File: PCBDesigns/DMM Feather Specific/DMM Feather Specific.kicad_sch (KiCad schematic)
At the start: 63 parts, among them J1 POWER2, J10 I_Input, J11 Conn_01x02_Pin, J12 Conn_01x02_Pin, J2 POWER1, J3 DIGITAL2, J4 Out to Screen, J5 ANALOG, J6 DIGITAL1, J7 Barrel_Jack, J8 Conn_01x01_Socket, J9 Barrel_Jack, Q1 MMBT3904, Q2 AO3400A MOSFET, Q3 AO3400A MOSFET, SW1 SW_Push, SW2 SW_Push, SW3 SW_Push, U1 RFM-0505S, U10 LM4040DBZ-2.5, U11 ADS1115IDGS, U2 ADuM1200AR, U3 ADuM1200AR, U4 ISO1540, U5 LM317_TO-220, U6 LM4040DBZ-5, U7 IX4426N, U8 MAX1683, U9 IX4426N

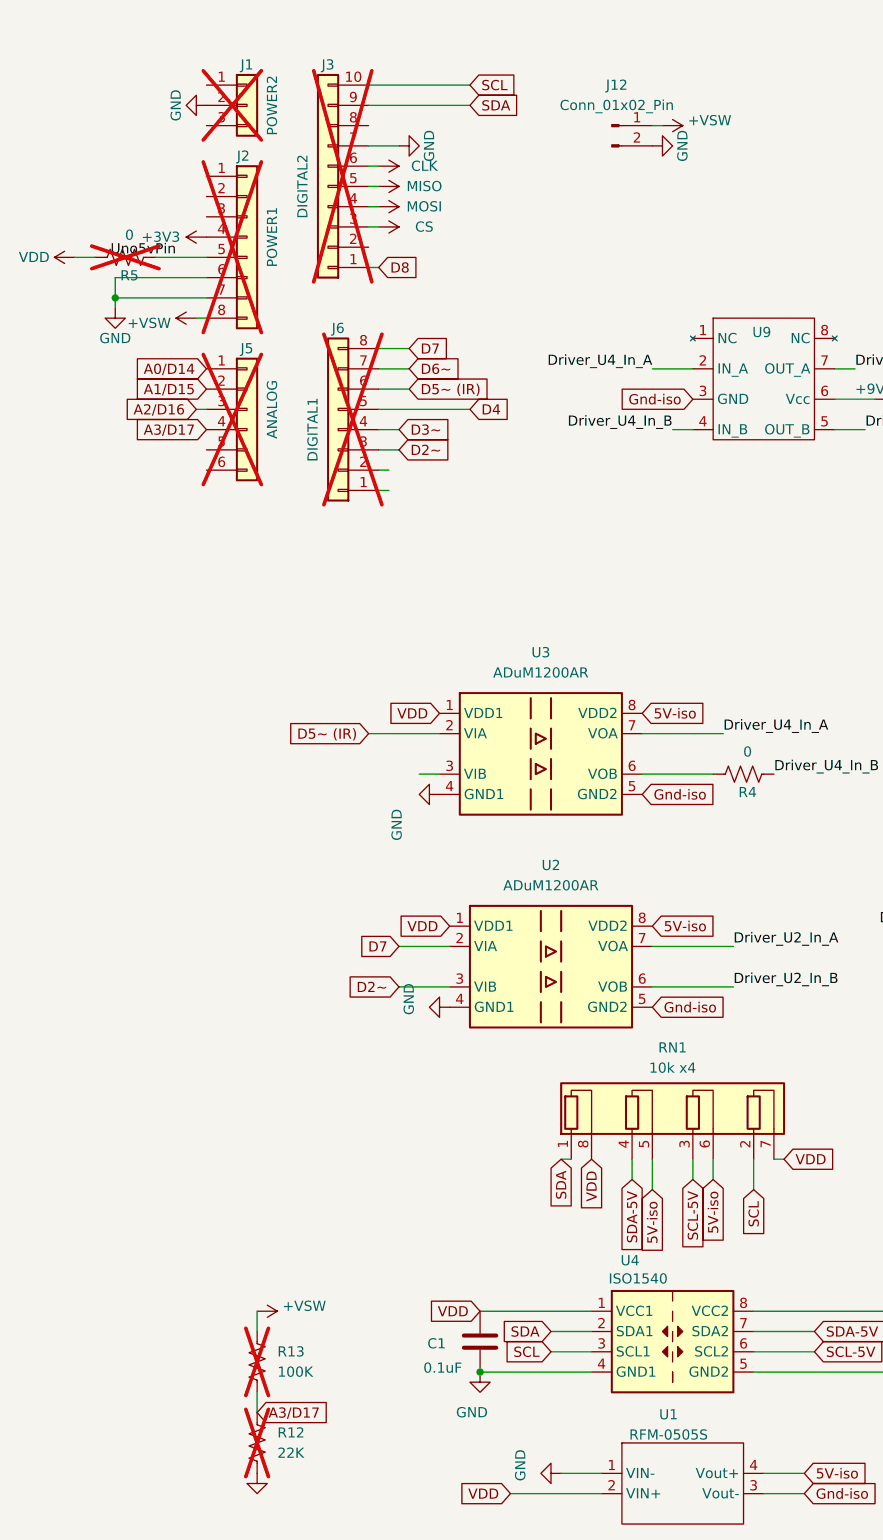
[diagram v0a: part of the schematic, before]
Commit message: Finished(?) an Uno footprint board, started on Feather specific
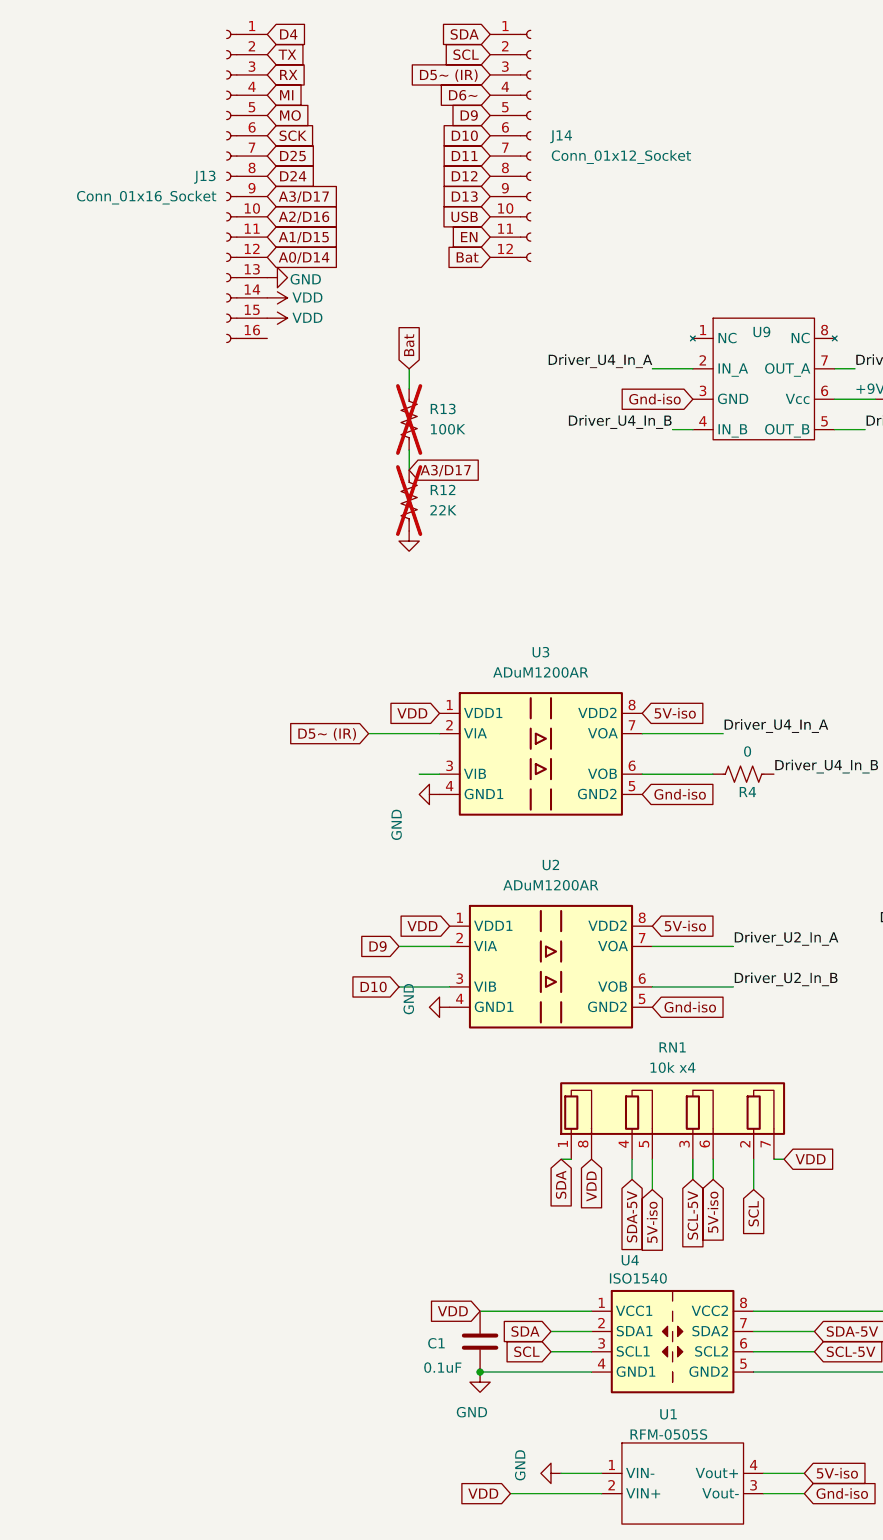
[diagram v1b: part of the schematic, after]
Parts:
- removed J1: POWER2, Library:PinHeader_1x03_P2.54mm_Vertical_NoBox, symbol Connector_Generic:Conn_01x03
- removed J12: Conn_01x02_Pin, Connector_PinSocket_2.54mm:PinSocket_1x02_P2.54mm_Vertical, symbol Connector:Conn_01x02_Pin
- removed J2: POWER1, Connector_PinHeader_2.54mm:PinHeader_1x08_P2.54mm_Vertical, symbol Connector_Generic:Conn_01x08
- removed J3: DIGITAL2, Connector_PinHeader_2.54mm:PinHeader_1x10_P2.54mm_Vertical, symbol Connector_Generic:Conn_01x10
- removed J5: ANALOG, Connector_PinHeader_2.54mm:PinHeader_1x06_P2.54mm_Vertical, symbol Connector_Generic:Conn_01x06
- removed J6: DIGITAL1, Connector_PinHeader_2.54mm:PinHeader_1x08_P2.54mm_Vertical, symbol Connector_Generic:Conn_01x08
- removed R5: 0, Resistor_SMD:R_0805_2012Metric_Pad1.20x1.40mm_HandSolder, symbol Device:R_US
- added J13: Conn_01x16_Socket, Connector_PinHeader_2.54mm:PinHeader_1x16_P2.54mm_Vertical, symbol Connector:Conn_01x16_Socket
- added J14: Conn_01x12_Socket, Connector_PinHeader_2.54mm:PinHeader_1x12_P2.54mm_Vertical, symbol Connector:Conn_01x12_Socket
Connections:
- net A0/D14: now also J13.12 (Pin_12)
- net A1/D15: now also J13.11 (Pin_11)
- net A2/D16: now also J13.10 (Pin_10)
- net A3/D17: now also J13.9 (Pin_9)
- net D4: now also J13.1 (Pin_1)
- net D5~ (IR): now also J14.3 (Pin_3)
- net D6~: now also J14.4 (Pin_4)
- net GND: now also J13.13 (Pin_13)
- net SCL: now also J14.2 (Pin_2)
- net SDA: now also J14.1 (Pin_1)
- net VDD: now also J13.14 (Pin_14), J13.15 (Pin_15)
- net +VSW renamed Bat
- net Bat: now also J14.12 (Pin_12)
- net D2~ renamed D10
- net D10: now also J14.6 (Pin_6)
- net D7 renamed D9
- net D9: now also J14.5 (Pin_5)
- new net D11: J14.7 (Pin_7)
- new net D12: J14.8 (Pin_8)
- new net D13: J14.9 (Pin_9)
- new net D24: J13.8 (Pin_8)
- new net D25: J13.7 (Pin_7)
- new net EN: J14.11 (Pin_11)
- new net MI: J13.4 (Pin_4)
- new net MO: J13.5 (Pin_5)
- new net RX: J13.3 (Pin_3)
- new net SCK: J13.6 (Pin_6)
- new net TX: J13.2 (Pin_2)
- new net USB: J14.10 (Pin_10)
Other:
- moved on the sheet: R12, R13
